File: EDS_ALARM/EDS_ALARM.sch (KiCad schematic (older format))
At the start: 24 parts, among them J1 USB_B_Micro, J2 Conn_01x06_Male, U1 STM32F411RETx, U2 CMWX1ZZABZ-078, U3 LT1117-3.3, Y1 Crystal

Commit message: Update EDS_ALARM.sch
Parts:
- added J3: 73412-0110, MOLEX_73412-0110, symbol U.FL:73412-0110
- PIR1: symbol EKMC1601111:EKMC1601111 -> EDS_ALARM-rescue:EKMC1601111-EKMC1601111
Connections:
- wire segments 65 -> 64
- no-connect marks 101 -> 58
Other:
- moved on the sheet: C13, C14, C15, C6, C7, J2, R1, R2, U1, Y1

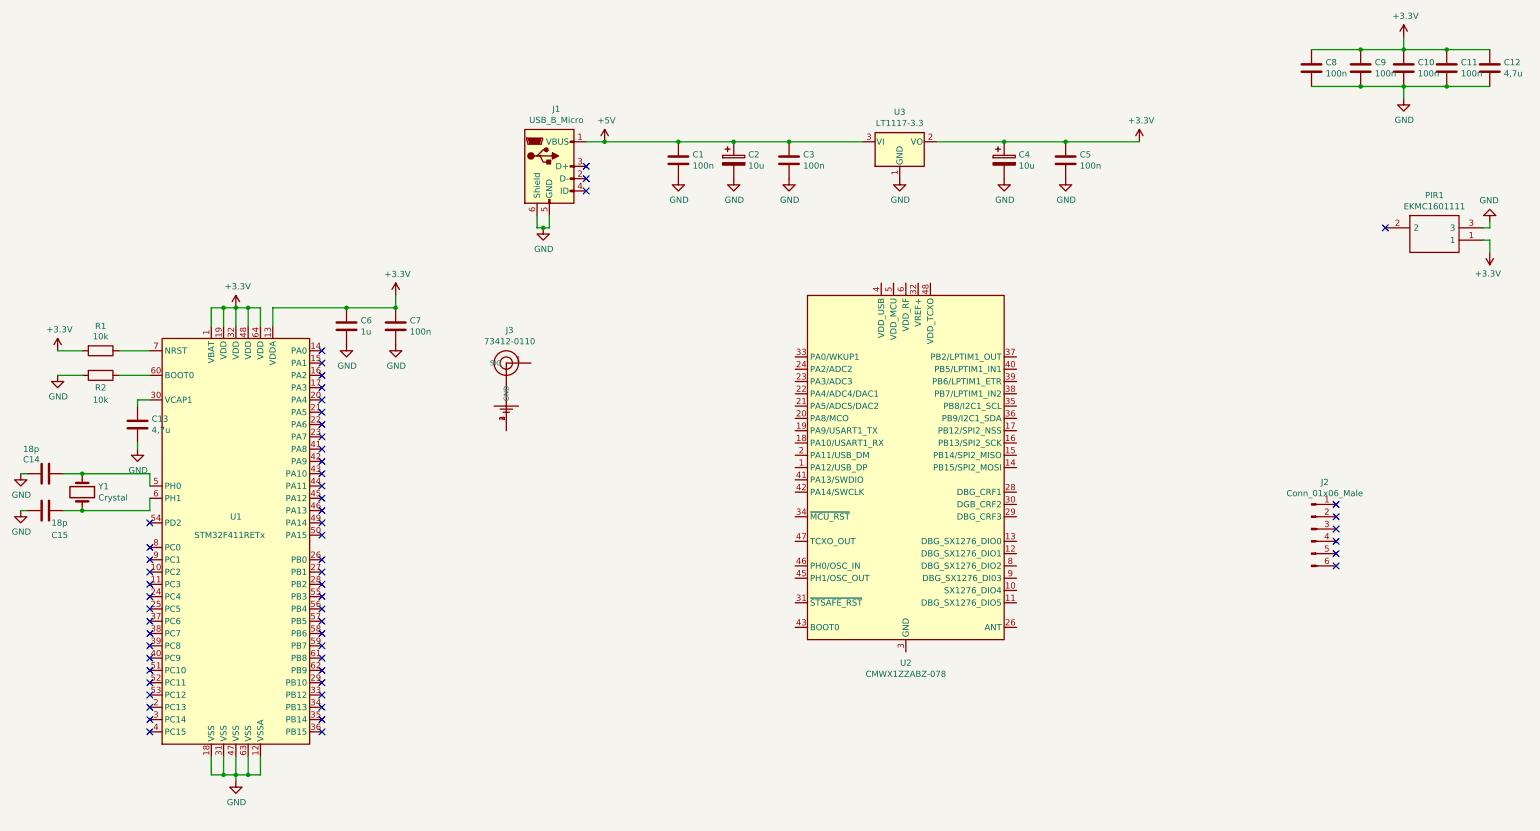
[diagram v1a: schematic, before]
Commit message: UPDATE
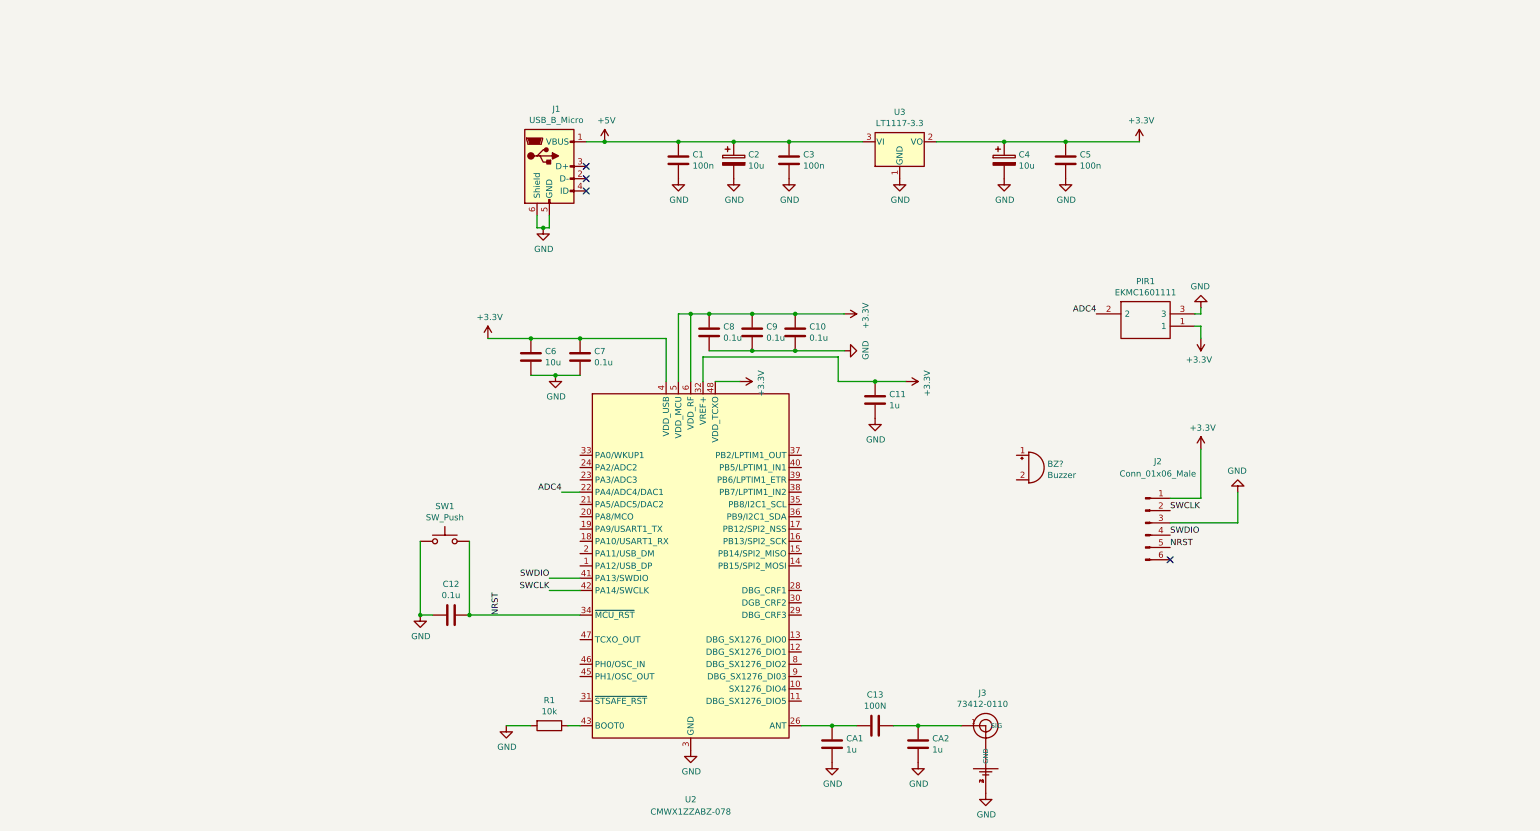
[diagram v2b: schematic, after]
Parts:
- removed C14, C15: 18p, symbol Device:C
- removed R2: 10k, symbol Device:R
- removed U1: STM32F411RETx, Package_QFP:LQFP-64_10x10mm_P0.5mm, symbol MCU_ST_STM32F4:STM32F411RETx
- removed Y1: Crystal, symbol Device:Crystal
- added BZ?: Buzzer, symbol Device:Buzzer
- added CA1, CA2: 1u, symbol Device:C
- added SW1: SW_Push, symbol Switch:SW_Push
- C10, C7, C8, C9: value 100n -> 0.1u
- C11: value 100n -> 1u
- C12: value 4,7u -> 0.1u
- C13: value 4,7u -> 100N
- C6: value 1u -> 10u
- J3: footprint MOLEX_73412-0110 -> Connector_Coaxial:U.FL_Molex_MCRF_73412-0110_Vertical
- PIR1: footprint VZ-STANDARD -> (none)
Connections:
- net +3V3: now also J2.1 (Pin_1), U2.32 (VREF+), U2.4 (VDD_USB), U2.48 (VDD_TCXO), U2.5 (VDD_MCU), U2.6 (VDD_RF); no longer C12.1, R1.2
- net GND: now also J2.3 (Pin_3), J3.2 (GND), J3.3 (GND), J3.4 (GND), R1.2, U2.25 (GND), U2.27 (GND), U2.3 (GND), U2.44 (GND), U2.49 (GND), U2.50 (GND), U2.51 (GND), U2.52 (GND), U2.53 (GND), U2.54 (GND), U2.55 (GND), U2.56 (GND), U2.57 (GND), U2.7 (GND), CA1.2, CA2.2, SW1.1; no longer C13.2
- net at C13.1: now also J3.1 (SIG), CA2.1
- net at R1.1: now also U2.43 (BOOT0)
- net SWCLK: now reaches J2.2 (Pin_2)
- net SWCLK: now also U2.42 (PA14/SWCLK)
- net SWDIO: now reaches J2.4 (Pin_4)
- net SWDIO: now also U2.41 (PA13/SWDIO)
- net NRST: now reaches J2.5 (Pin_5)
- net NRST: now also C12.1, U2.34 (~MCU_RST), SW1.2
- net ADC4: now reaches U2.22 (PA4/ADC4/DAC1)
- net ADC4: now also PIR1.2
- net at U2.26 (ANT): now also C13.2, CA1.1
- no-connect marks 58 -> 4
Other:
- moved on the sheet: J2, J3, PIR1, U2
